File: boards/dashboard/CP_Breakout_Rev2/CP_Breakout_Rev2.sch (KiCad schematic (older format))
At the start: 17 parts, among them J1 Conn_01x06, J2 Conn_01x02, J3 Conn_01x06, U1 LM2936-3.3, U2 CP2120

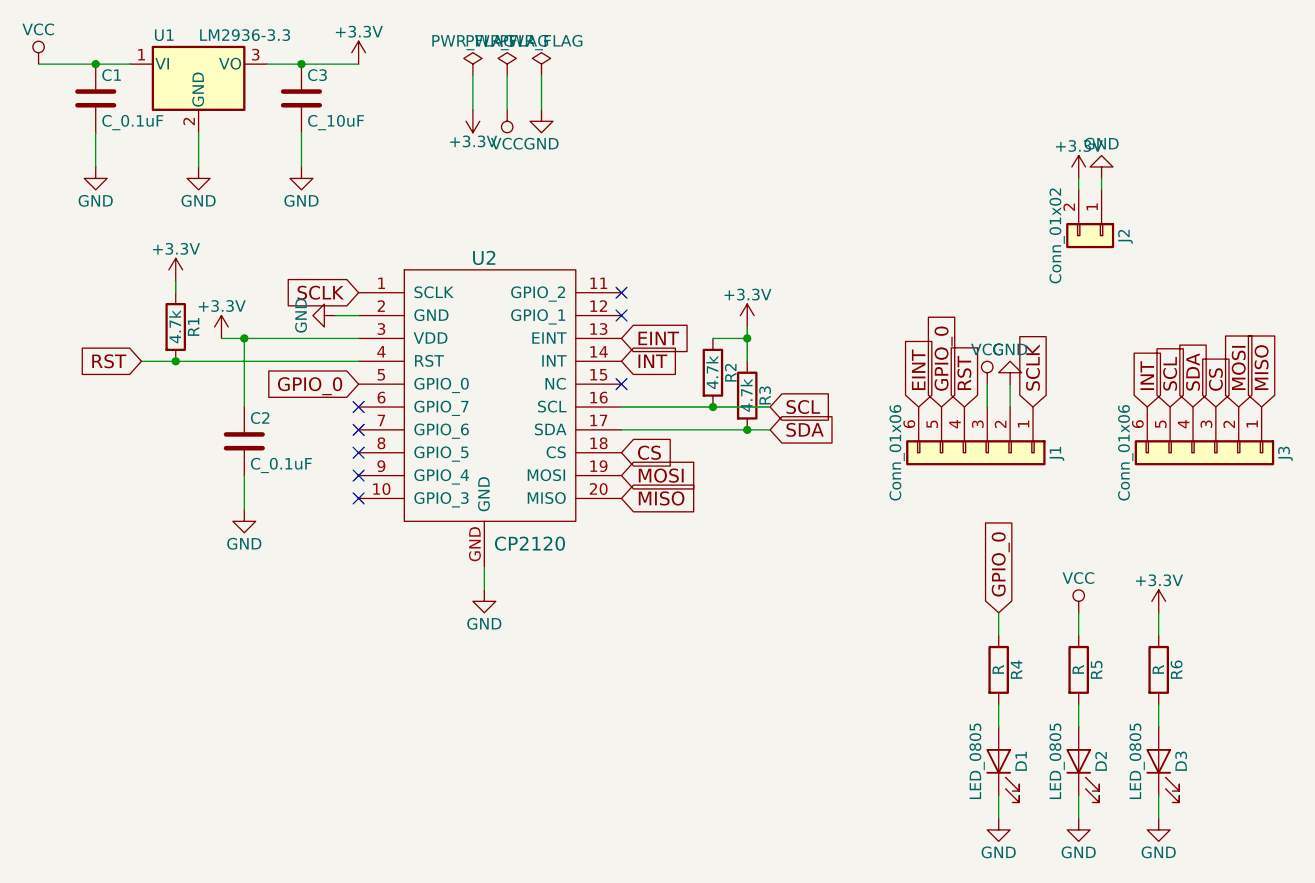
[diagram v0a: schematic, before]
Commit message: Revisions to CP2120 board files
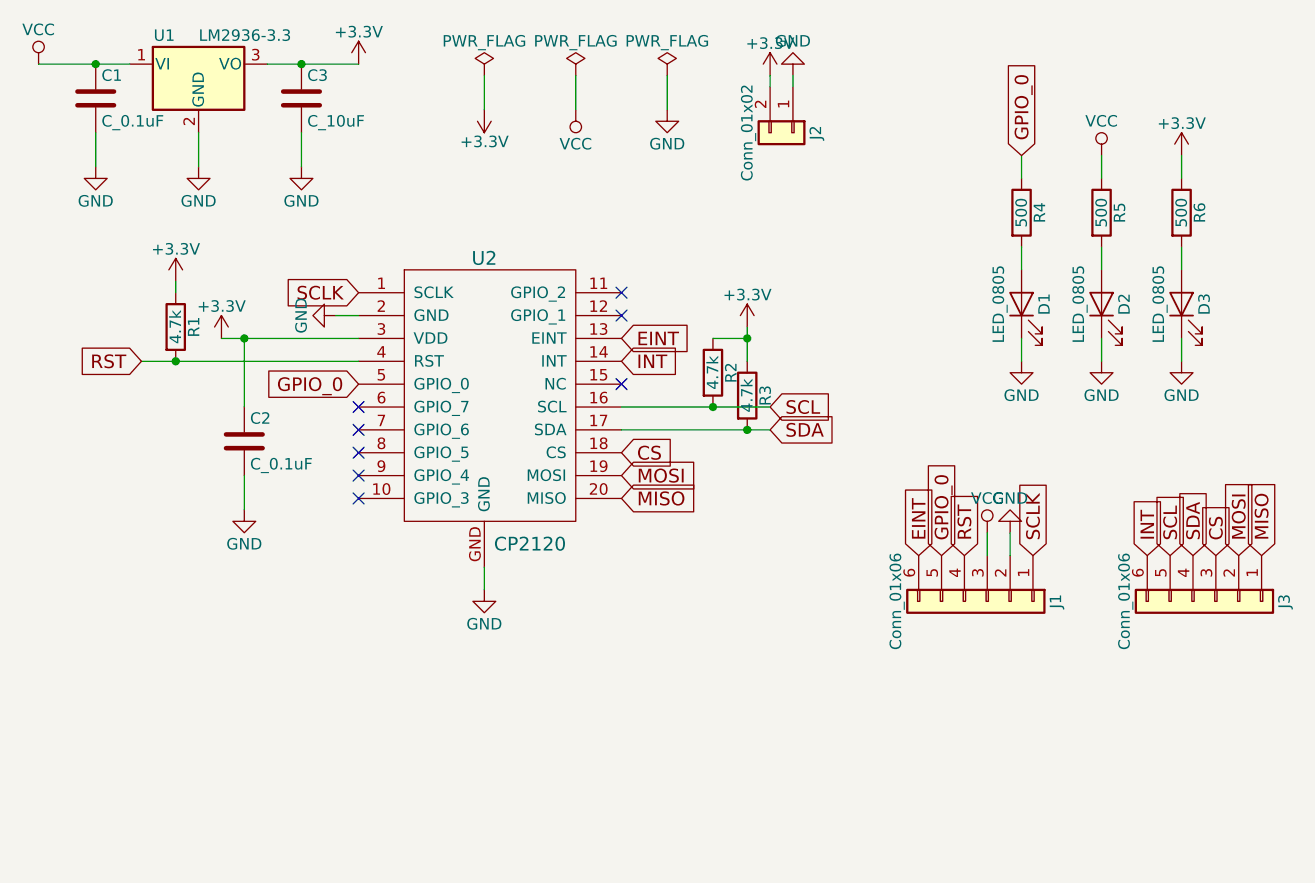
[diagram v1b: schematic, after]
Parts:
- R4, R5, R6: value R -> 500
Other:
- moved on the sheet: D1, D2, D3, J1, J2, J3, R4, R5, R6
